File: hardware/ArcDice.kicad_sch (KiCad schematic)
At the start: 22 parts, among them J1 SW ON/OFF, SW2 SW_Push, U1 ATtiny13A-P, U2 TP4056_Module

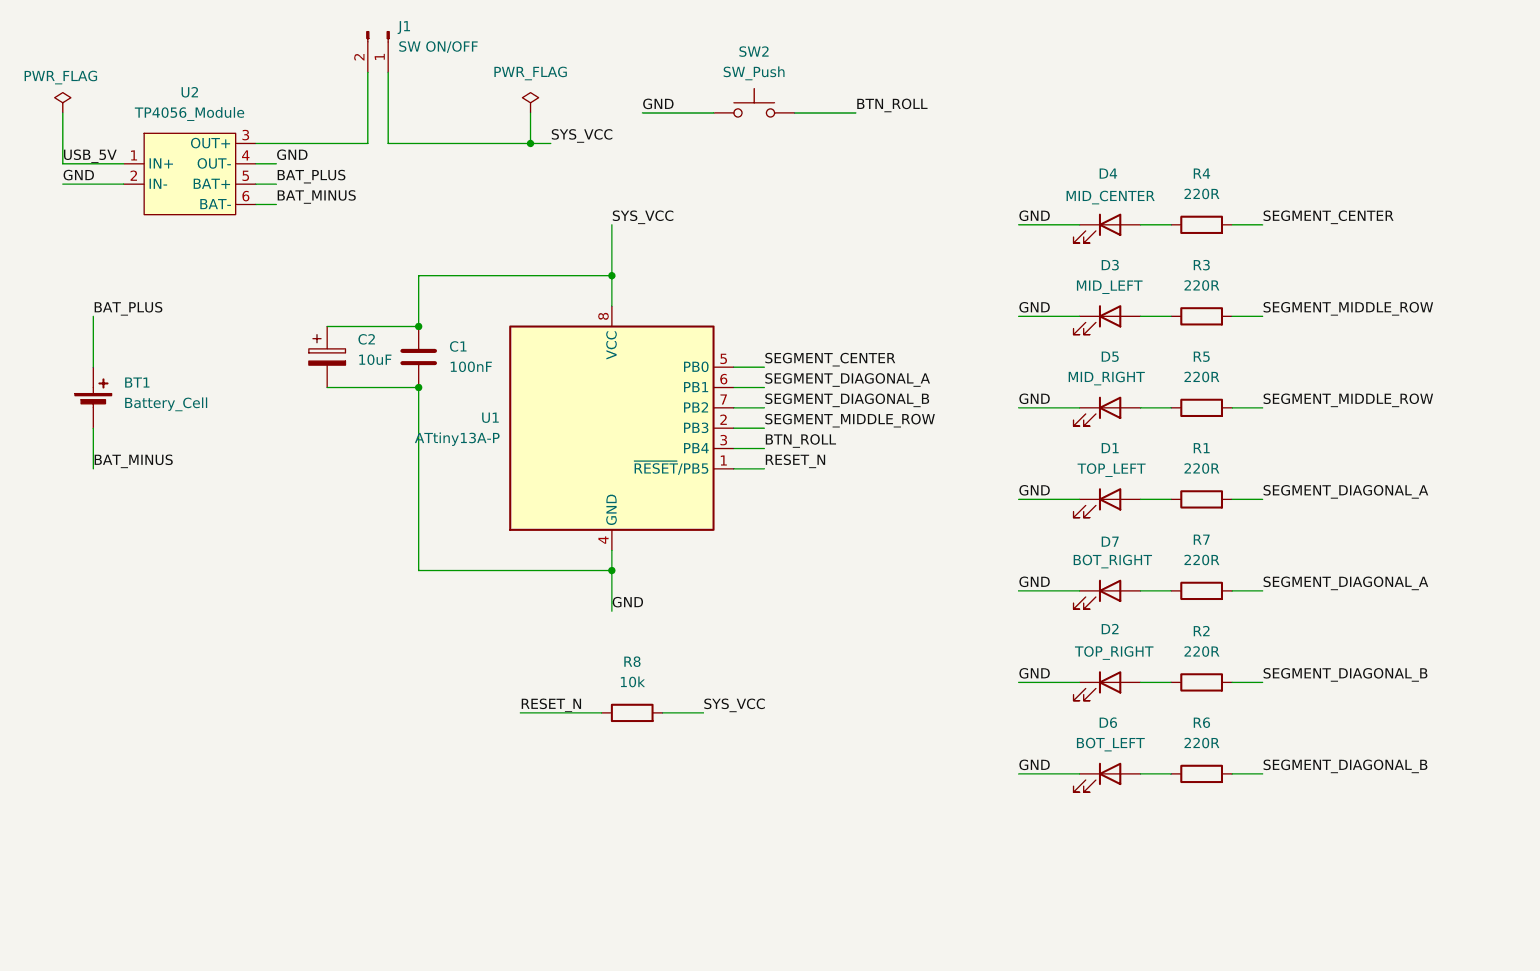
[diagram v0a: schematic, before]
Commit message: Update ArcDice project files
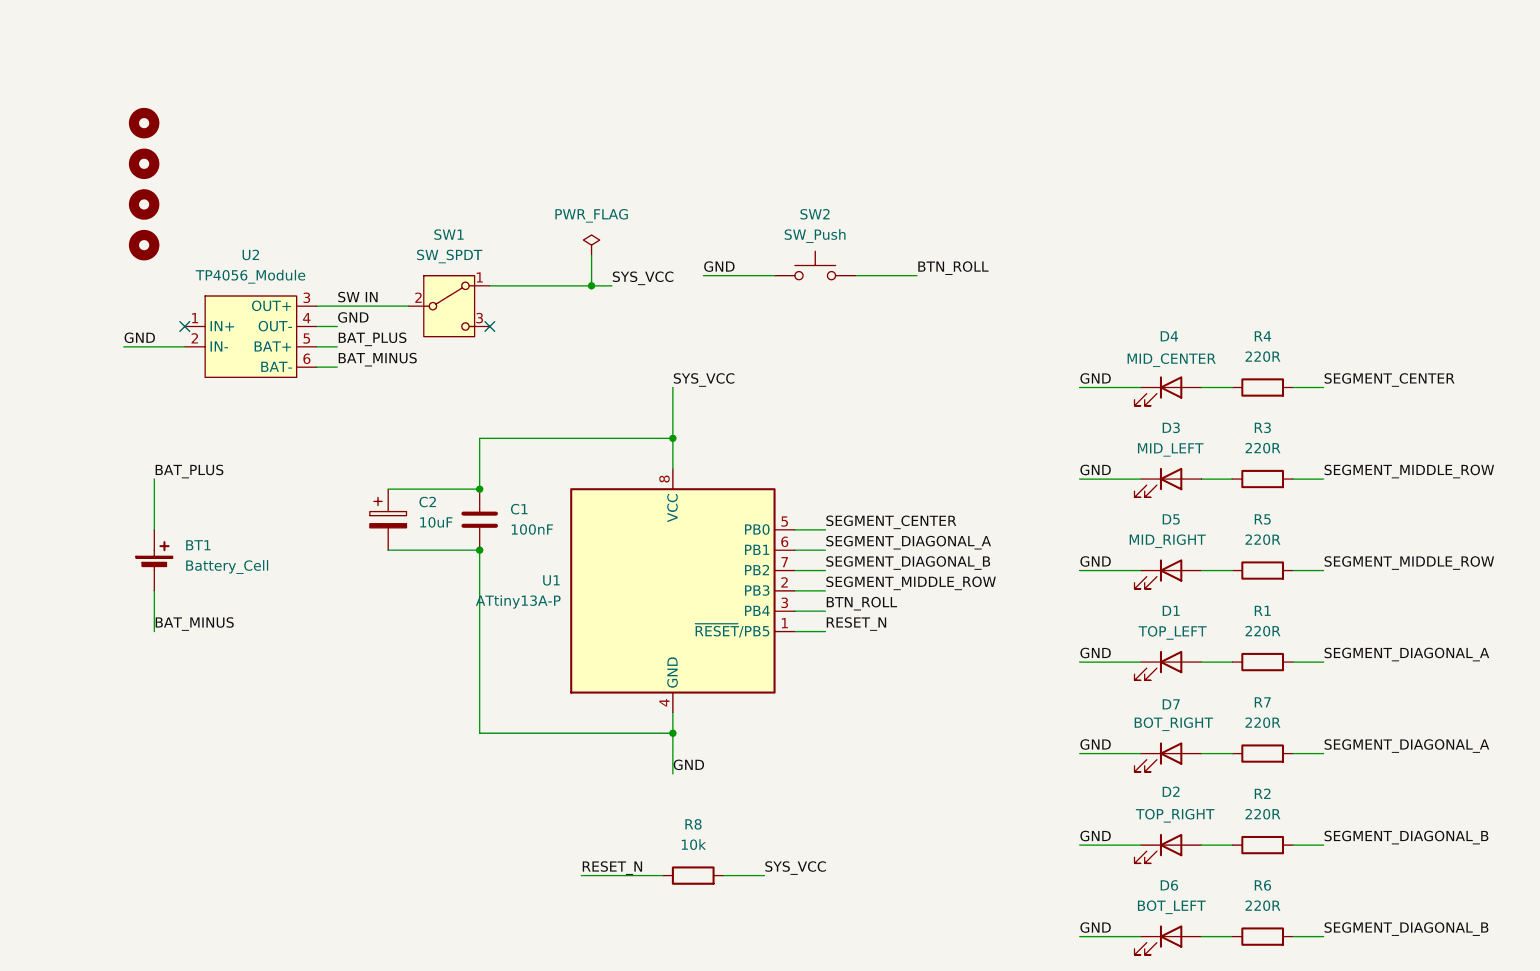
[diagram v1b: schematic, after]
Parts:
- removed J1: SW ON/OFF, Connector_JST:JST_PH_B2B-PH-K_1x02_P2.00mm_Vertical, symbol Connector:Conn_01x02_Pin
- added H1, H2, H3, H4: MountingHole, MountingHole:MountingHole_2.2mm_M2, symbol Mechanical:MountingHole
- added SW1: SW_SPDT, Button_Switch_THT:Switch_Slide_SS12D06_Generic, symbol Switch:SW_SPDT
- BT1: footprint (none) -> Battery:Battery_18250_Tabbed_1S
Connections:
- net SYS_VCC: now also SW1.1 (A)
- net SW IN: now reaches U2.3 (OUT+)
- net SW IN: now also SW1.2 (B)
- net USB_5V: no longer names the net of U2.1 (IN+)
- no-connect marks 0 -> 2
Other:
- title: Digital Dice -> ArcDice
- moved on the sheet: BT1, C1, C2, D1, D2, D3, D4, D5, D6, D7, R1, R2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

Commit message: hardware: update KiCad schematic, PCB, and project files
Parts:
- H1, H2, H3, H4: footprint MountingHole:MountingHole_2.2mm_M2 -> MountingHole:MountingHole_3.2mm_M3
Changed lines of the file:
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@@
 	(title_block
 		(title "ArcDice")
-		(date "2026-07-12")
-		(rev "v1.0")
+		(date "2026-09-11")
+		(rev "v1.1")
 		(company "MM Industries")
 	)
@@
 			)
 		)
-		(property "Footprint" "MountingHole:MountingHole_2.2mm_M2"
+		(property "Footprint" "MountingHole:MountingHole_3.2mm_M3"
 			(at 63.5 44.45 0)
 			(hide yes)
@@
 			)
 		)
-		(property "Footprint" "MountingHole:MountingHole_2.2mm_M2"
+		(property "Footprint" "MountingHole:MountingHole_3.2mm_M3"
 			(at 63.5 54.61 0)
 			(hide yes)
@@
 			)
 		)
-		(property "Footprint" "MountingHole:MountingHole_2.2mm_M2"
+		(property "Footprint" "MountingHole:MountingHole_3.2mm_M3"
 			(at 63.5 39.37 0)
 			(hide yes)
@@
 			)
 		)
-		(property "Footprint" "MountingHole:MountingHole_2.2mm_M2"
+		(property "Footprint" "MountingHole:MountingHole_3.2mm_M3"
 			(at 63.5 49.53 0)
 			(hide yes)
